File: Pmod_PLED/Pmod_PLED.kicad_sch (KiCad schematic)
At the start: 7 parts, among them IC1 TBD62064APG, IC2 LM2940T-5.0, J1 Barrel_Jack_Switch, J2 Conn_01x06_Pin, J3 Conn_01x03_Pin

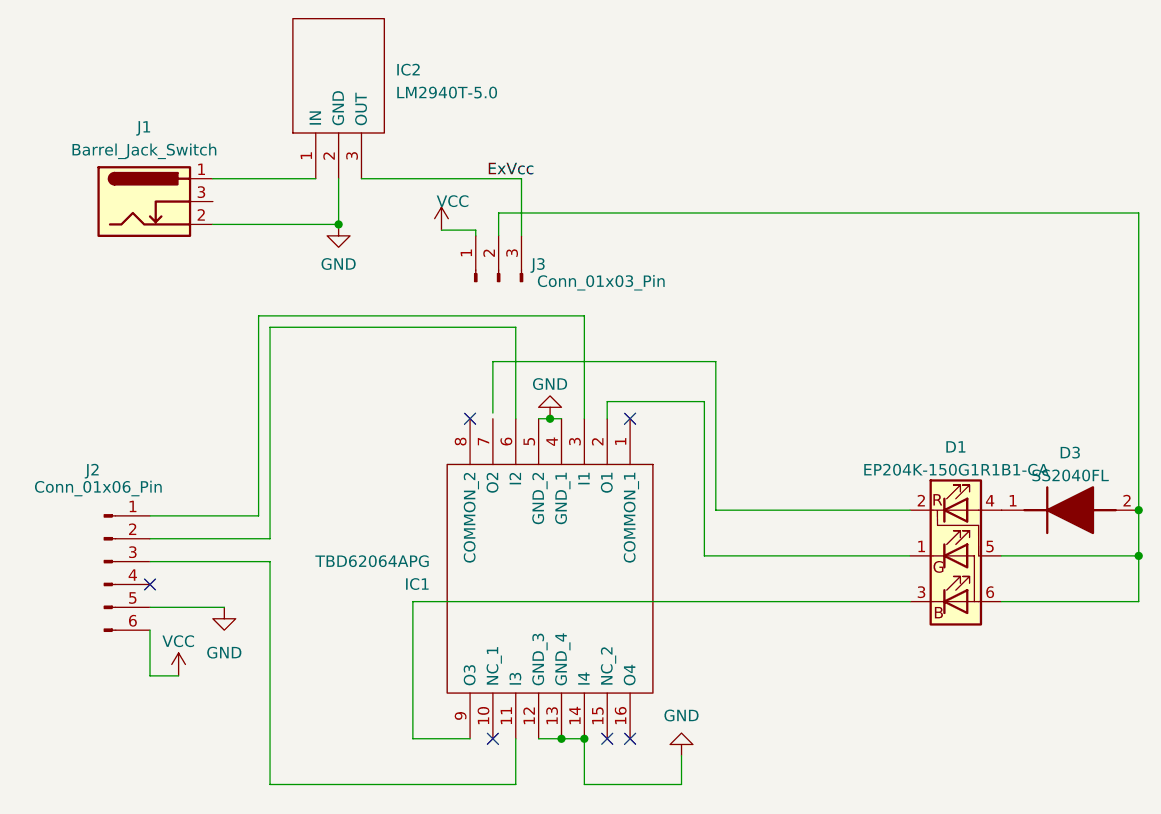
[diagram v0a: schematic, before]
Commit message: 30
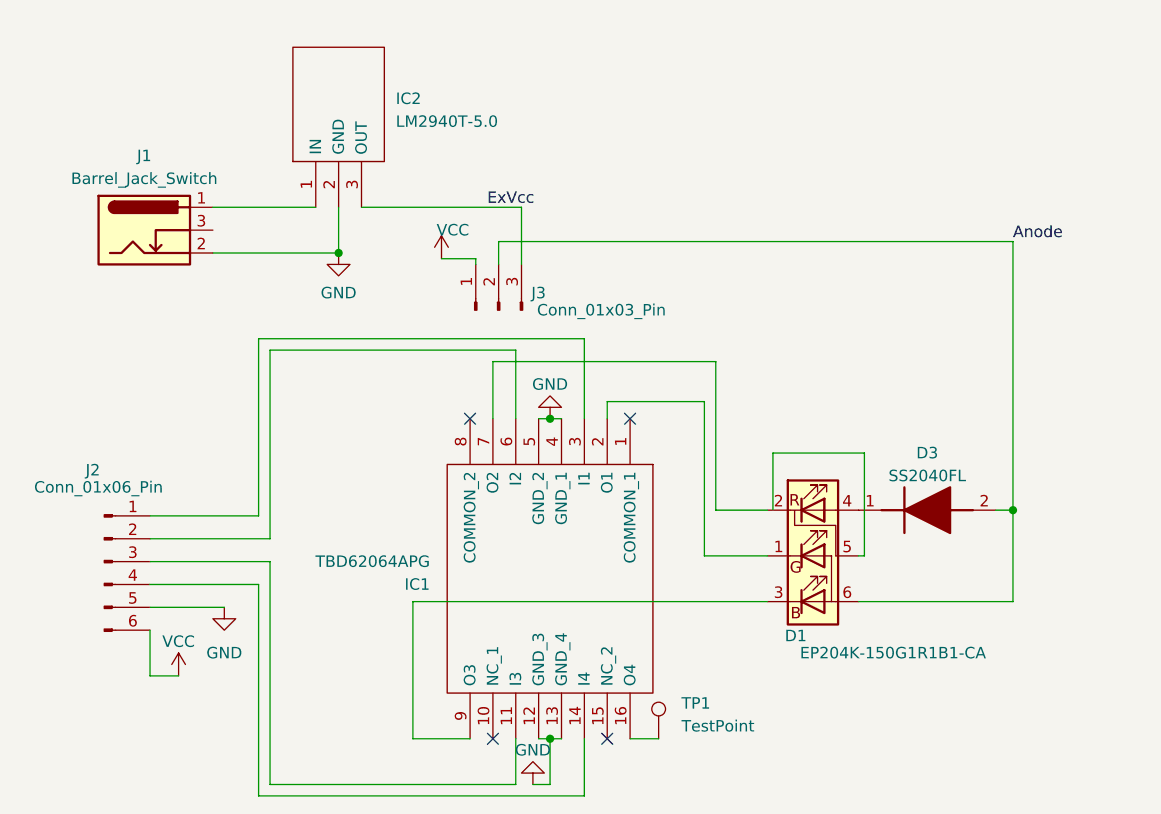
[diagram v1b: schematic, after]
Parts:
- added TP1: TestPoint, TestPoint:TestPoint_Pad_D2.0mm, symbol Connector:TestPoint
- J2: footprint Connector_PinHeader_2.54mm:PinHeader_1x06_P2.54mm_Vertical -> Library:Pmod6
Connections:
- net GND: no longer IC1.14 (I4)
- net Anode: now reaches D1.6 (A), D3.2 (A), J3.2 (Pin_2)
- net Anode: no longer D1.5 (RK)
- net at J2.4 (Pin_4): now also IC1.14 (I4)
- net at D1.2 (RK): now also IC1.7 (O2)
- net at IC1.16 (O4): now also TP1.1
- no-connect marks 6 -> 4
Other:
- moved on the sheet: D1, D3, IC2, J1, J3
